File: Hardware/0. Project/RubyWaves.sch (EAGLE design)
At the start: 62 parts, among them CN1 USB 3.2 Gen 2 Type C Receptac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, CN2 Lithium Ion Polymer, J2 CORTEX_DEBUGPTH, Q2 SI2374DS, Q3 SI2374DS, U1 MAX32664, U2 MAX30102, U3 MT3608, U4 NRF52832, U5 MCP73831/2, U6 S-8261ACMMD-G4MT2U, Y1 32MHz, Y2 32.768kHz, Y3 32.768 kHz

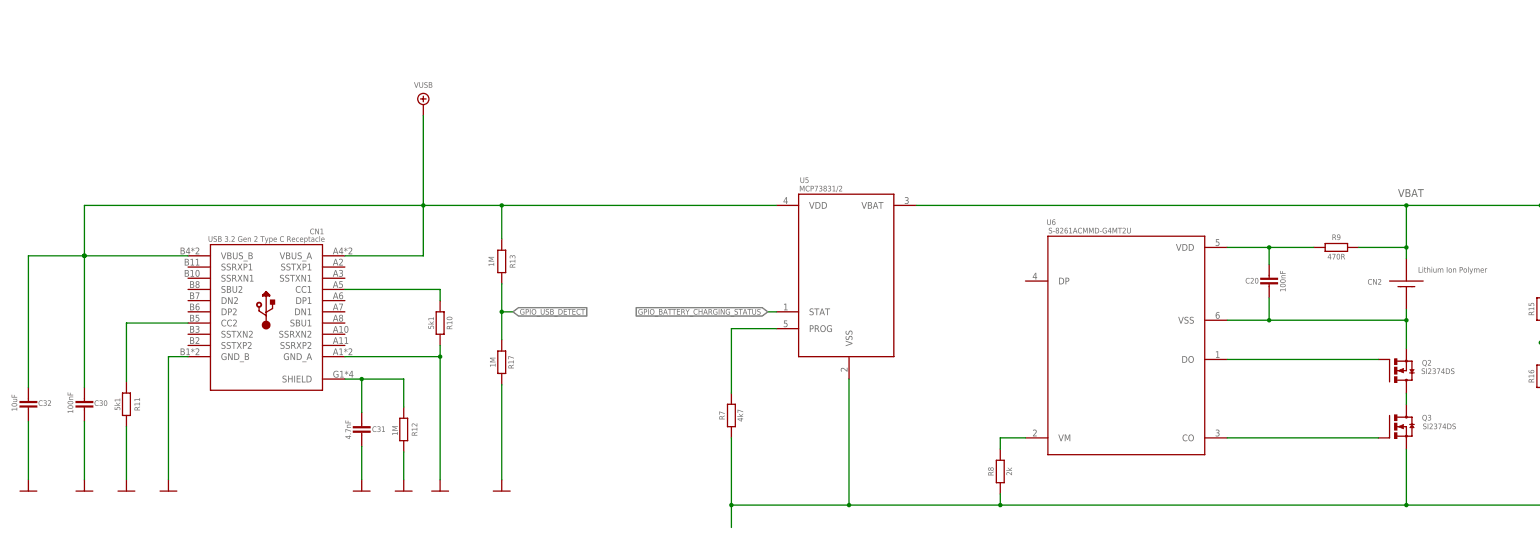
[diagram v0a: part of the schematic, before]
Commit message: New board reference added
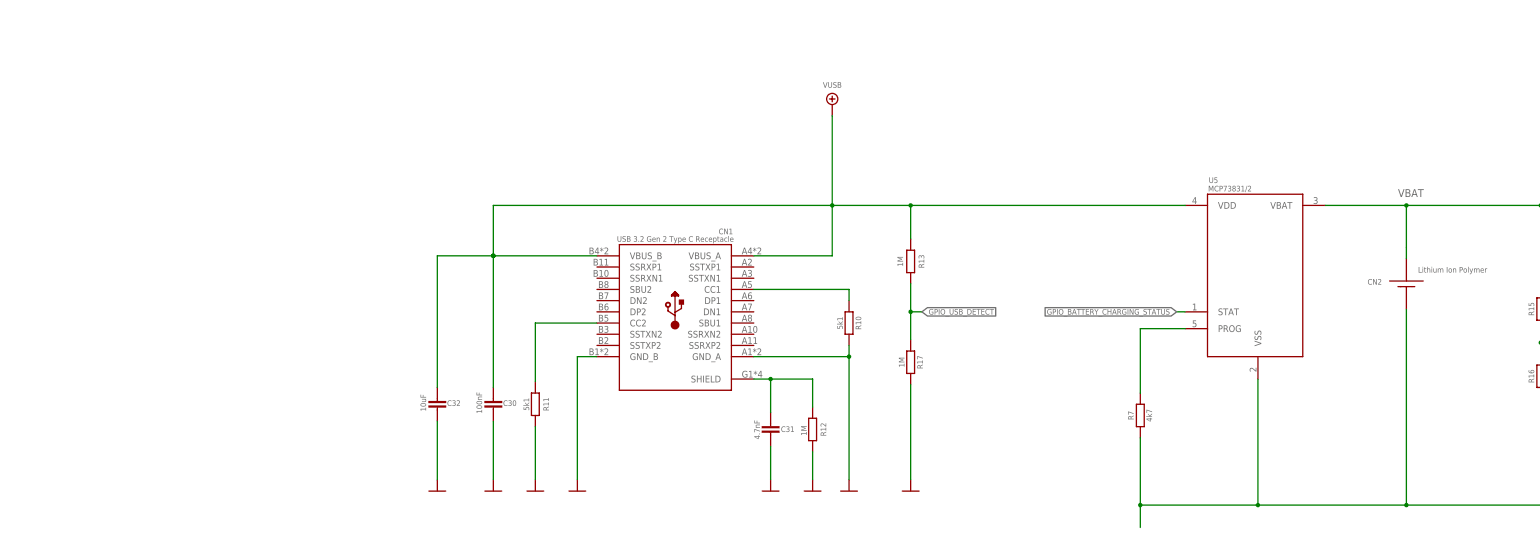
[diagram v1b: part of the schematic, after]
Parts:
- removed C20: 100nF, My-RLC:C_0603
- removed Q2, Q3: SI2374DS, SI2374DS:SI2374DSSOT23
- removed R8: 2k, My-RLC:R_0603
- removed R9: 470R, My-RLC:R_0603
- removed U6: S-8261ACMMD-G4MT2U, SamacSys_Parts:S-8261ACMMD-G4MT2U
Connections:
- removed net N$27: Q3.G, U6.CO
- removed net N$29: R8.2, U6.VM
- removed net N$31: C20.1, R9.2, U6.VDD
- removed net N$32: C20.2, CN2.GND, Q2.S, U6.VSS
- removed net N$7: Q2.G, U6.DO
- removed net N$9: Q2.D, Q3.D
- net 0V1: now also CN2.GND; no longer Q3.S, R8.1
- net VBAT: no longer R9.1
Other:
- note removed: "7μA max."
- note removed: "Overcharge = 4.325V"
- note removed: "Overdischarge = 3.000V"
- moved on the sheet: C30, C31, C32, CN1, R10, R11, R12, R13, R17, R7, U5
